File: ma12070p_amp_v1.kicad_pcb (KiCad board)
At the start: 2 copper layers, 105 x 85 mm, 81 parts, among them J1 Screw_Terminal_01x02, J2 Screw_Terminal_01x04, U1 TPS62175DQC, U2 MA12070P

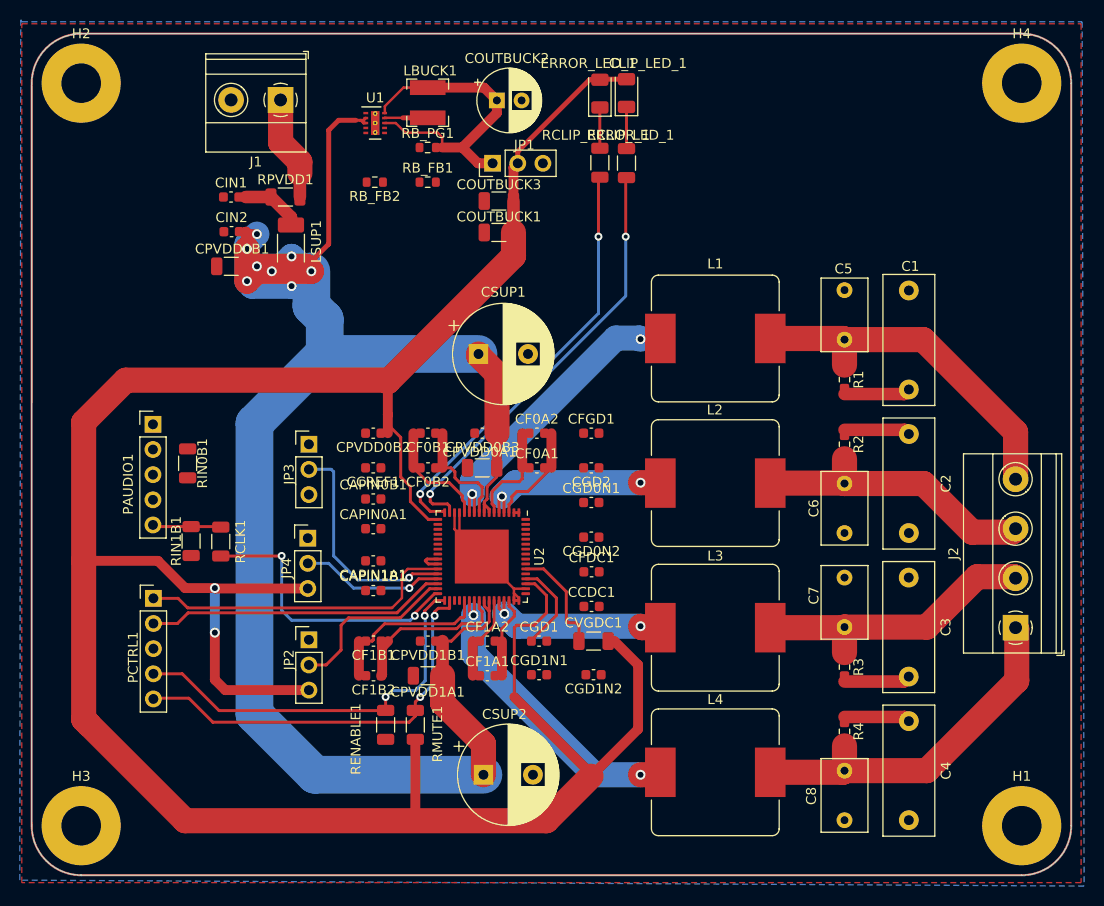
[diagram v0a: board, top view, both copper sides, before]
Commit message: Revert "update"
This reverts commit 23222dc2ff684dbeb0c499af5827ef2ca36430f4.
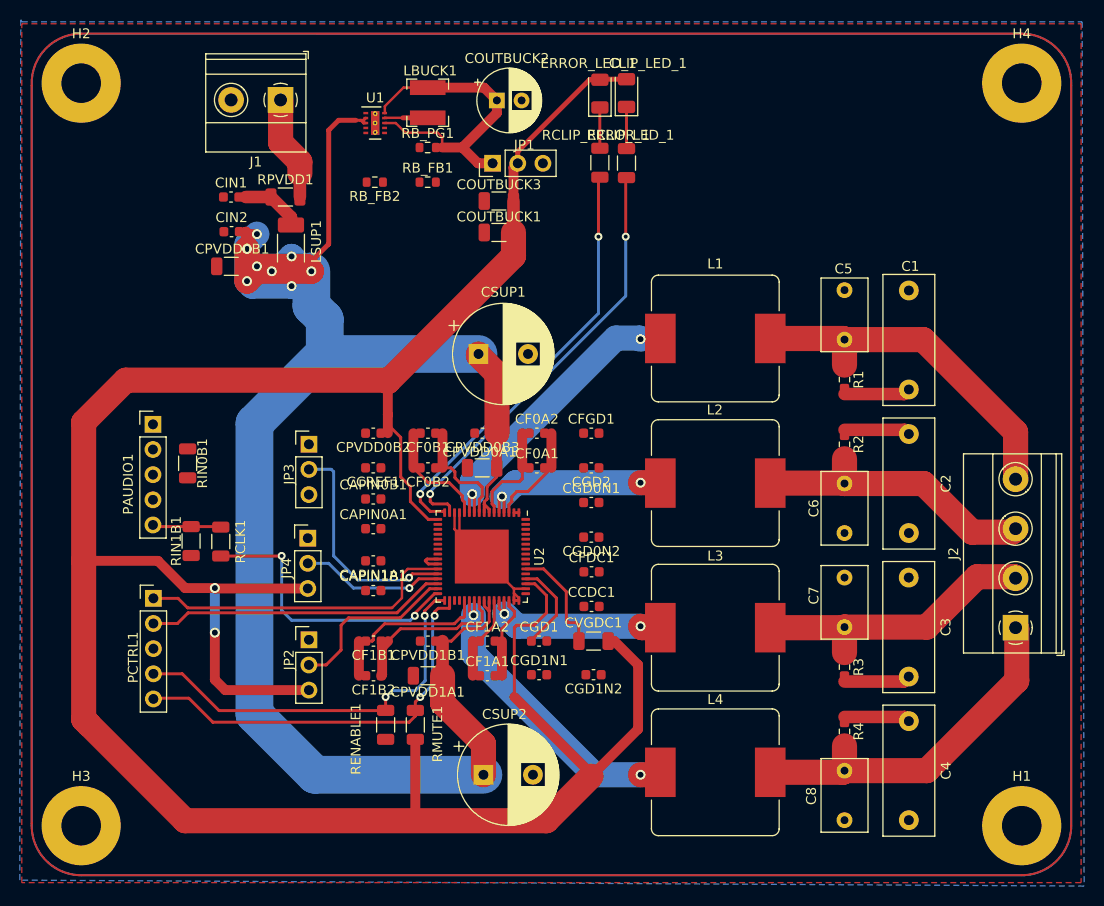
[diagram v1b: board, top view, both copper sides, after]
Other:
- board outline removed
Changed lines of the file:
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@@
   (gr_arc (start 110.005659 50.244072) (mid 111.381359 46.555821) (end 115 45.006246) (layer "B.Cu") (width 0.2))
   (gr_arc (start 215 124.756246) (mid 213.712311 128.365003) (end 210.25 130.006246) (layer "B.Cu") (width 0.2))
-  (gr_line (start 215 50) (end 215 125) (layer "Edge.Cuts") (width 0.05))
-  (gr_line (start 110 125) (end 110 50) (layer "Edge.Cuts") (width 0.05))
-  (gr_arc (start 110 50) (mid 111.464466 46.464466) (end 115 45) (layer "Edge.Cuts") (width 0.05))
-  (gr_arc (start 115 130) (mid 111.464466 128.535534) (end 110 125) (layer "Edge.Cuts") (width 0.05))
-  (gr_line (start 210 130) (end 115 130) (layer "Edge.Cuts") (width 0.05))
-  (gr_line (start 115 45) (end 210 45) (layer "Edge.Cuts") (width 0.05))
-  (gr_arc (start 210 45) (mid 213.535534 46.464466) (end 215 50) (layer "Edge.Cuts") (width 0.05))
-  (gr_arc (start 215 125) (mid 213.535534 128.535534) (end 210 130) (layer "Edge.Cuts") (width 0.05))
-  (gr_rect (start 109 44) (end 216 131) (layer "F.CrtYd") (width 0.05) (fill none))
   (segment (start 152.71 95.065) (end 152.71 93.3775) (width 0.25) (layer "F.Cu") (net 1))
   (segment (start 151.0225 98.065) (end 149.935 98.065) (width 0.3) (layer "F.Cu") (net 1))

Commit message: update
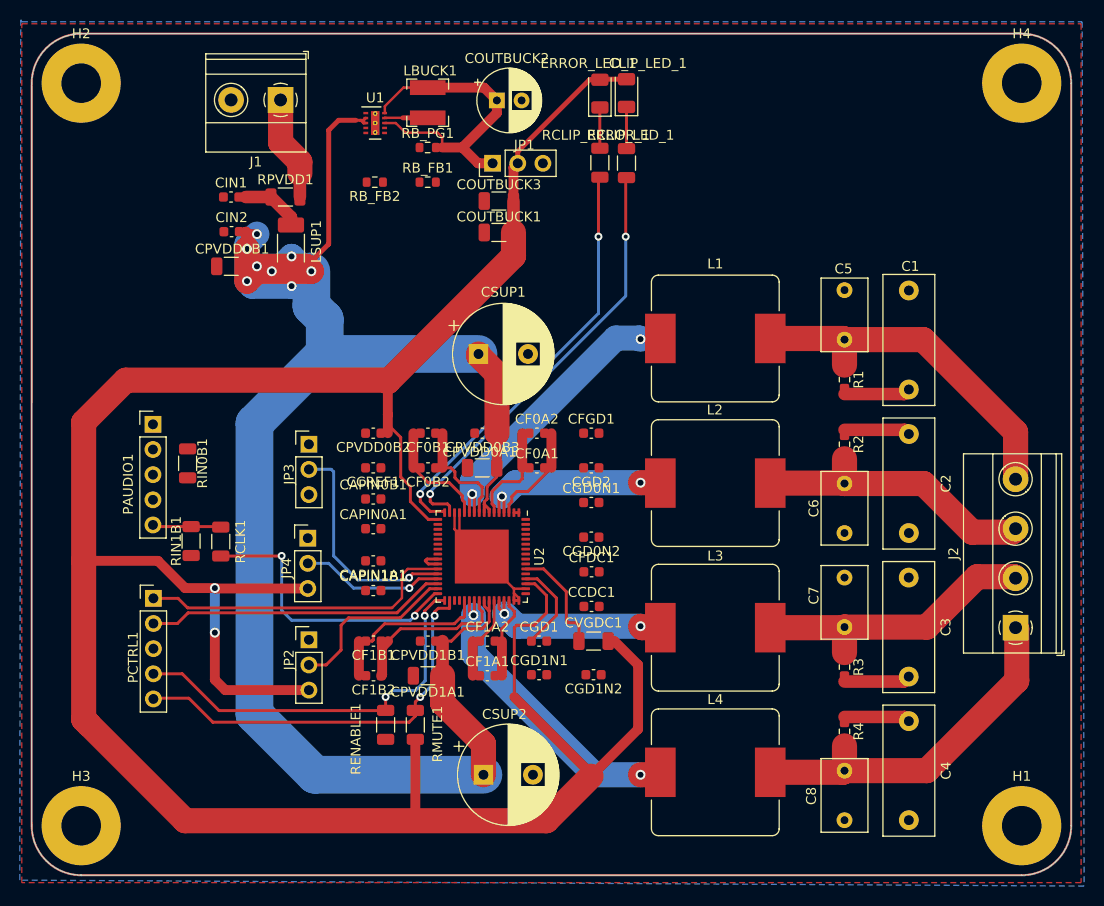
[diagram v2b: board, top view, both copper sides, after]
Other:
- board outline added: 105 x 85 mm
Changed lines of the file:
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@@
   (gr_arc (start 110.005659 50.244072) (mid 111.381359 46.555821) (end 115 45.006246) (layer "B.Cu") (width 0.2))
   (gr_arc (start 215 124.756246) (mid 213.712311 128.365003) (end 210.25 130.006246) (layer "B.Cu") (width 0.2))
+  (gr_line (start 215 50) (end 215 125) (layer "Edge.Cuts") (width 0.05))
+  (gr_line (start 110 125) (end 110 50) (layer "Edge.Cuts") (width 0.05))
+  (gr_arc (start 110 50) (mid 111.464466 46.464466) (end 115 45) (layer "Edge.Cuts") (width 0.05))
+  (gr_arc (start 115 130) (mid 111.464466 128.535534) (end 110 125) (layer "Edge.Cuts") (width 0.05))
+  (gr_line (start 210 130) (end 115 130) (layer "Edge.Cuts") (width 0.05))
+  (gr_line (start 115 45) (end 210 45) (layer "Edge.Cuts") (width 0.05))
+  (gr_arc (start 210 45) (mid 213.535534 46.464466) (end 215 50) (layer "Edge.Cuts") (width 0.05))
+  (gr_arc (start 215 125) (mid 213.535534 128.535534) (end 210 130) (layer "Edge.Cuts") (width 0.05))
+  (gr_rect (start 109 44) (end 216 131) (layer "F.CrtYd") (width 0.05) (fill none))
   (segment (start 152.71 95.065) (end 152.71 93.3775) (width 0.25) (layer "F.Cu") (net 1))
   (segment (start 151.0225 98.065) (end 149.935 98.065) (width 0.3) (layer "F.Cu") (net 1))
